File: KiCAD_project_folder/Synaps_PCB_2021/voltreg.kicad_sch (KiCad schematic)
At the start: 12 parts, among them U8 AP63203WU-7, U9 AP63205WU-7

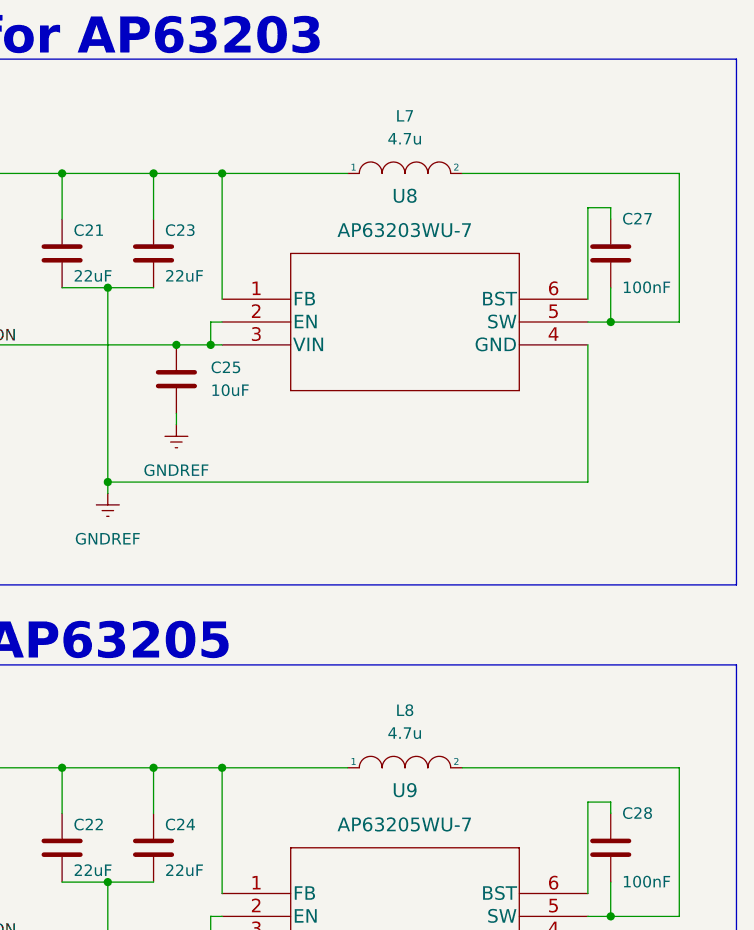
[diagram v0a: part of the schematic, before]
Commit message: schematic finished
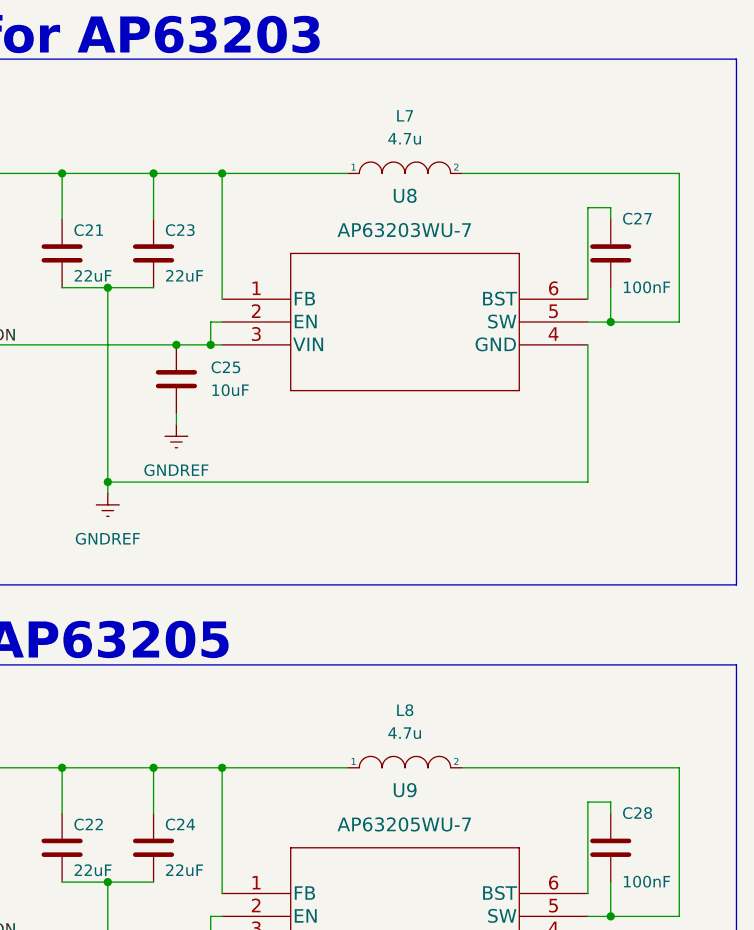
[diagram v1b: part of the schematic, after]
